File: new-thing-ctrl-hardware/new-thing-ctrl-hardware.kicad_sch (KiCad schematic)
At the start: 43 parts, among them J1 MSTBAish, J10 MSTBAish, J11 Neopixels, J2 MSTBAish, J3 SD, J4 MFRC522, J5 Conn_01x04_Male, J6 Screw_Terminal_01x09, J7 LCD, J8 Screw_Terminal_01x06, J9 Screw_Terminal_01x06, Q1 TIP120, Q2 TIP120, SW1 6X6, SW2 6X6, SW3 6X6, SW4 6X6, U1 L7805, U2 Pico

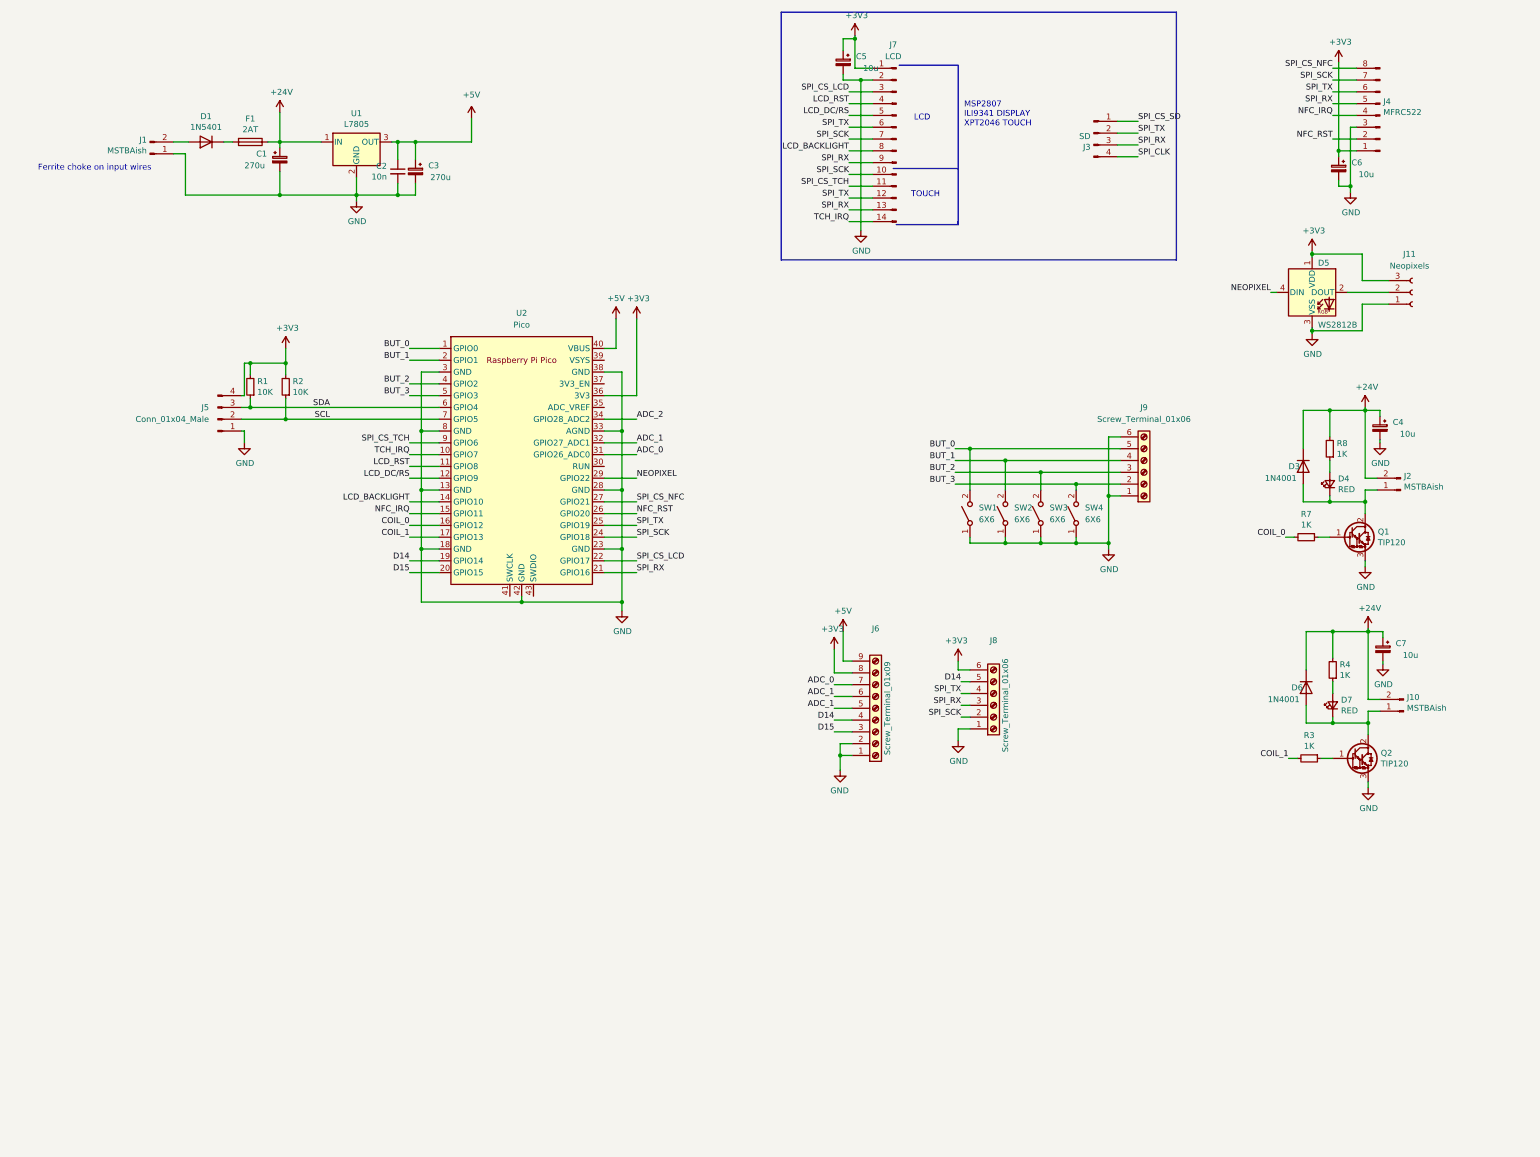
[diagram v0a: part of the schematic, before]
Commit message: routed
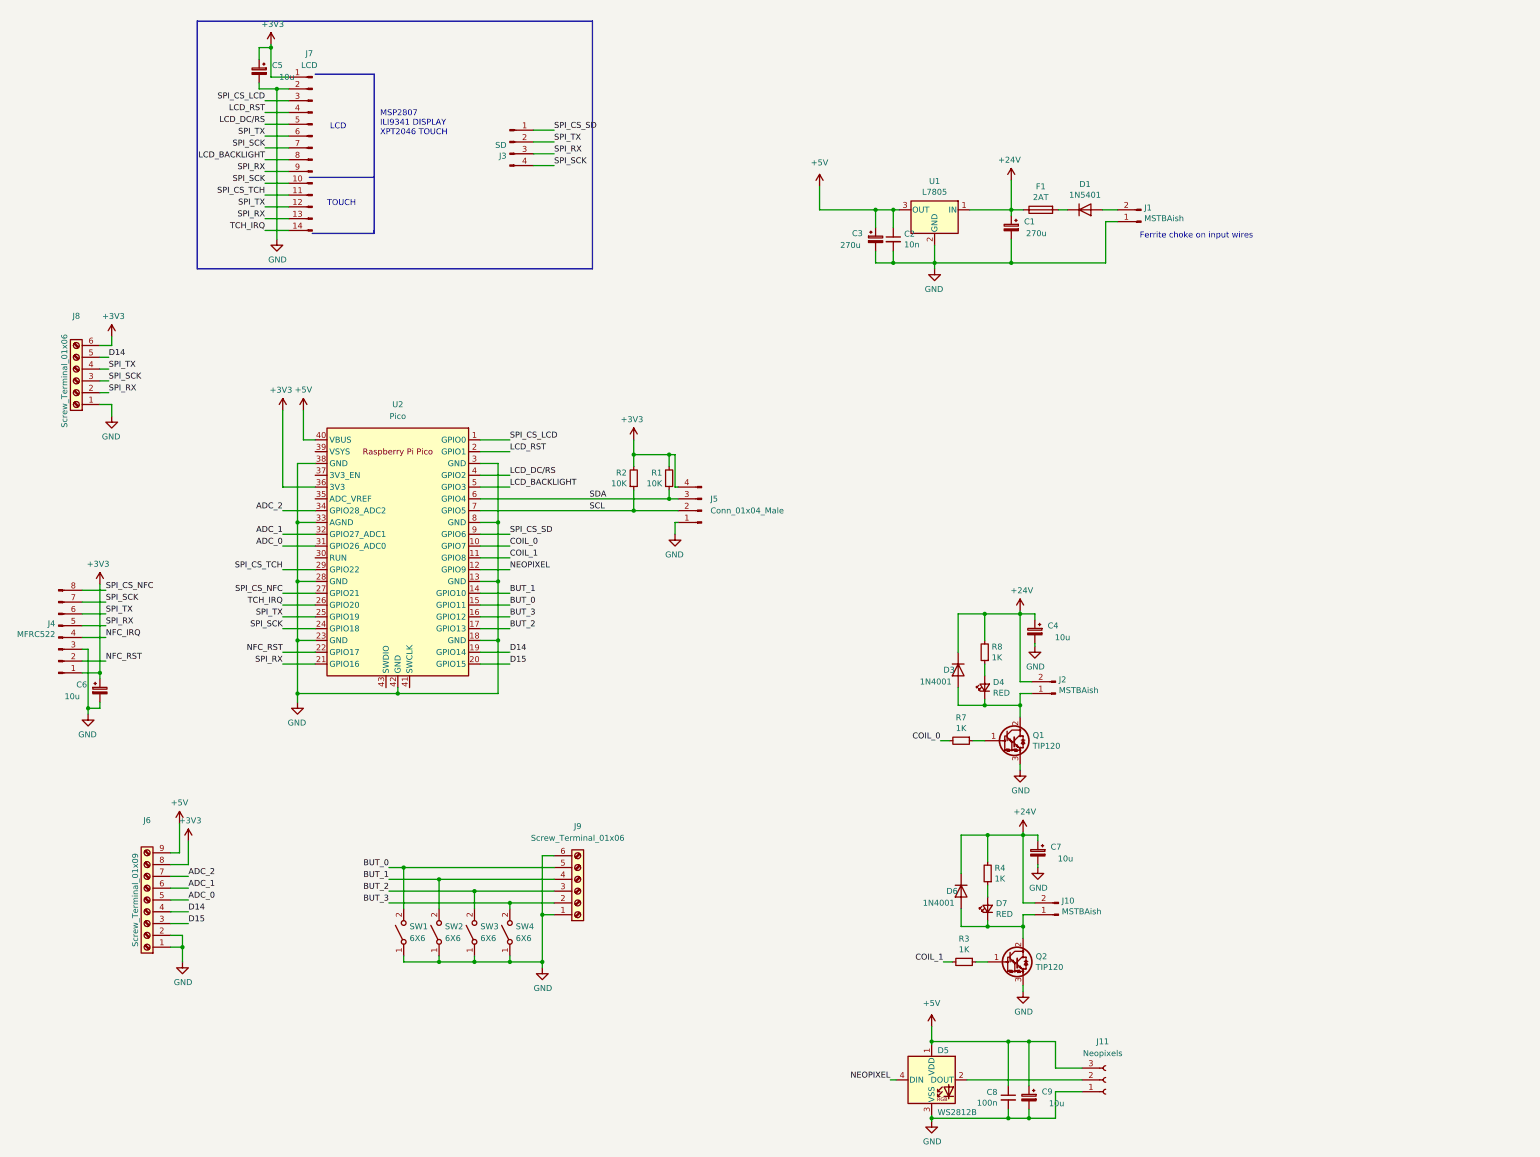
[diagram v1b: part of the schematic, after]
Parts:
- added C8: 100n, Capacitor_THT:C_Disc_D7.0mm_W2.5mm_P5.00mm, symbol Device:C_Small
- added C9: 10u, Capacitor_THT:CP_Radial_D5.0mm_P2.50mm, symbol machine-controller-rescue:CP_Small-Device
- SW1, SW2, SW3, SW4: footprint Button_Switch_THT:SW_PUSH_6mm_H7.3mm -> Button_Switch_THT:SW_PUSH_6mm_H13mm
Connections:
- net SPI_CLK is gone; now on net SPI_SCK: J3.4 (Pin_4)
- net +3V3: no longer D5.1 (VDD), J11.3 (Pin_3)
- net +5V: now also D5.1 (VDD), J11.3 (Pin_3), C8.1, C9.1
- net ADC_0: now also J6.5 (Pin_5); no longer J6.7 (Pin_7)
- net ADC_1: no longer J6.5 (Pin_5)
- net ADC_2: now also J6.7 (Pin_7)
- net BUT_0: now also U2.15 (GPIO11); no longer U2.1 (GPIO0)
- net BUT_1: now also U2.14 (GPIO10); no longer U2.2 (GPIO1)
- net BUT_2: now also U2.17 (GPIO13); no longer U2.4 (GPIO2)
- net BUT_3: now also U2.16 (GPIO12); no longer U2.5 (GPIO3)
- net COIL_0: now also U2.10 (GPIO7); no longer U2.16 (GPIO12)
- net COIL_1: now also U2.11 (GPIO8); no longer U2.17 (GPIO13)
- net GND: now also C8.2, C9.2
- net LCD_BACKLIGHT: now also U2.5 (GPIO3); no longer U2.14 (GPIO10)
- net LCD_DC/RS: now also U2.4 (GPIO2); no longer U2.12 (GPIO9)
- net LCD_RST: now also U2.2 (GPIO1); no longer U2.11 (GPIO8)
- net NEOPIXEL: now also U2.12 (GPIO9); no longer U2.29 (GPIO22)
- net NFC_IRQ: no longer U2.15 (GPIO11)
- net NFC_RST: now also U2.22 (GPIO17); no longer U2.26 (GPIO20)
- net SPI_CS_LCD: now also U2.1 (GPIO0); no longer U2.22 (GPIO17)
- net SPI_CS_SD: now also U2.9 (GPIO6)
- net SPI_CS_TCH: now also U2.29 (GPIO22); no longer U2.9 (GPIO6)
- net SPI_RX: now also J8.2 (Pin_2); no longer J8.3 (Pin_3)
- net SPI_SCK: now also J8.3 (Pin_3); no longer J8.2 (Pin_2)
- net TCH_IRQ: now also U2.26 (GPIO20); no longer U2.10 (GPIO7)
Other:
- moved on the sheet: C1, C2, C3, C4, C5, C6, C7, D1, D3, D4, D5, D6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
